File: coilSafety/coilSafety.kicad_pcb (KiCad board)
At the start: 2 copper layers, 99.1 x 99.1 mm, 22 parts, among them J1 PJ-037BH, J10 Conn_01x02_Pin, J11 Conn_01x02_Pin, J2 Screw_Terminal_01x08, J3 Screw_Terminal_01x02, J4 Screw_Terminal_01x02, J5 Screw_Terminal_01x06, J6 Screw_Terminal_01x02, J7 Conn_01x01_Pin, J8 Conn_01x08_Pin, J9 Conn_01x02_Pin, K1 AZ943-1CH-12DE

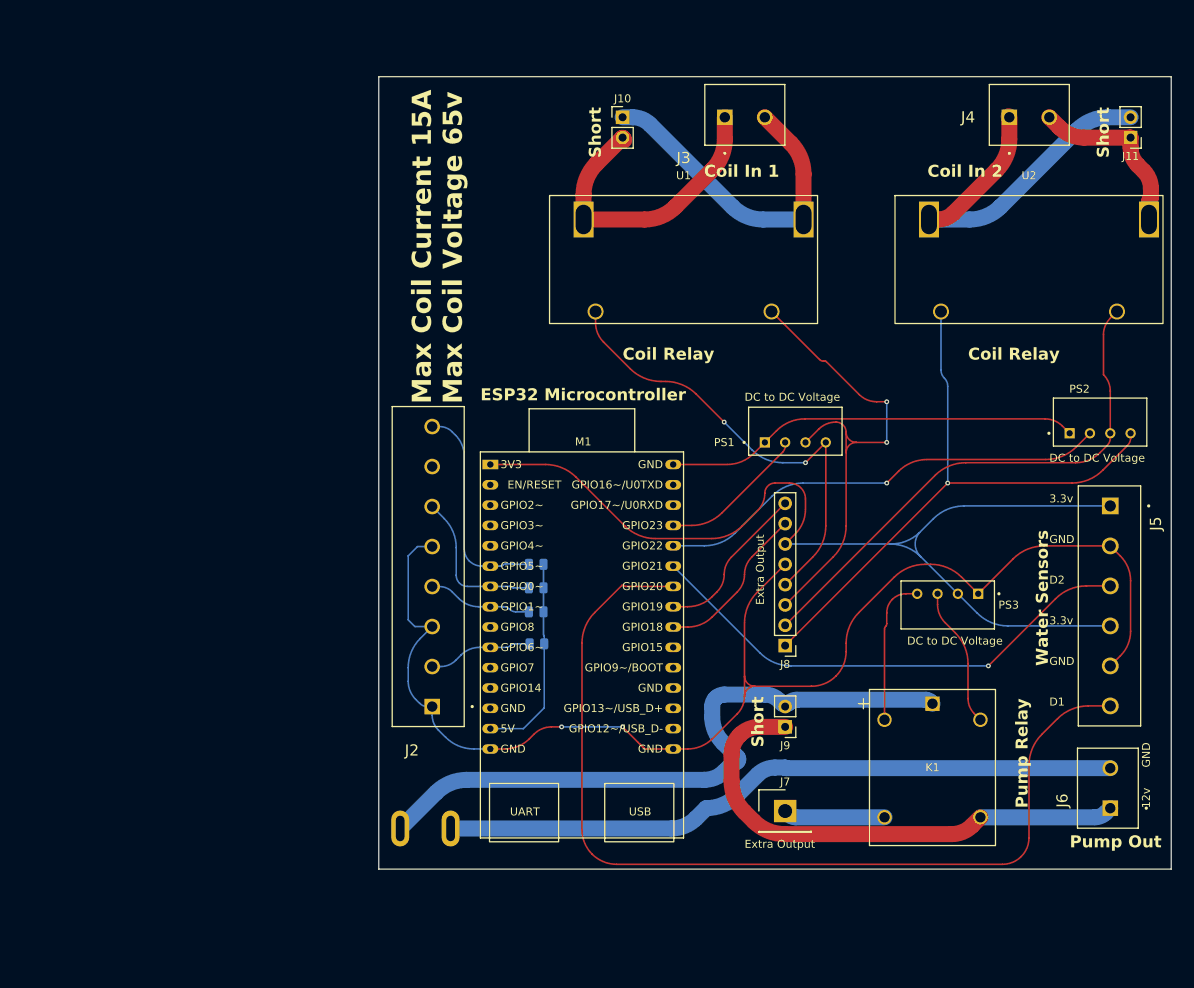
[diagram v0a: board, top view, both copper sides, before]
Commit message: Working on PCB
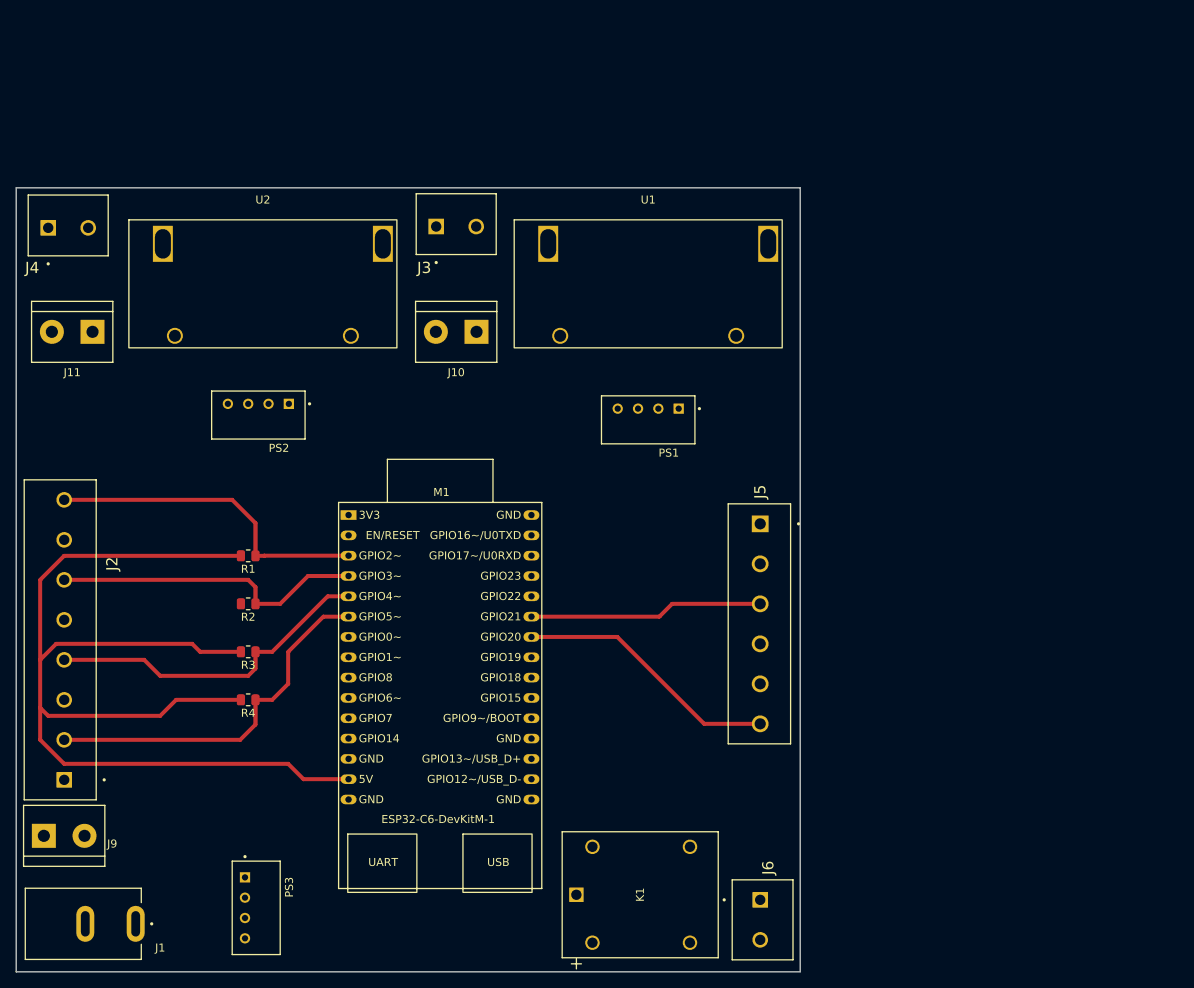
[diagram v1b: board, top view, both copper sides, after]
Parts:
- removed J7: Conn_01x01_Pin, Connector_Samtec_HPM_THT:Samtec_HPM-01-01-x-S_Straight_1x01_Pitch5.08mm
- removed J8: Conn_01x08_Pin, Connector_PinHeader_2.54mm:PinHeader_1x08_P2.54mm_Vertical
- J1, R1, R2, R3, R4: moved to F.Cu
- J10, J11, J9: footprint Connector_PinHeader_2.54mm:PinHeader_1x02_P2.54mm_Vertical -> TerminalBlock:TerminalBlock_bornier-2_P5.08mm
- M1: value ~ -> ESP32-C6-DevKitM-1
- U1, U2: value ~ -> AZDC007-1AE-12D
- moved J11 132.0 mm to (111.5, 70.0)
- moved J4 120.9 mm to (106.0, 57.0)
- moved PS2 105.2 mm to (132.3, 80.4), turned to 180 degrees
- moved U2 95.8 mm to (132.8, 64.0)
- moved PS3 94.4 mm to (132.0, 142.0), turned to -90 degrees
- moved J9 93.7 mm to (105.5, 133.0), turned to 0 degrees
- moved K1 50.5 mm to (172.0, 140.4), turned to 90 degrees
- moved J2 46.9 mm to (108.0, 126.0)
- moved J6 45.2 mm to (195.0, 141.0), turned to -90 degrees
- moved J5 43.8 mm to (195.0, 94.0)
- moved J3 38.6 mm to (154.5, 56.8)
- moved R4 36.8 mm to (131.0, 116.0), turned to 180 degrees
- moved R3 36.3 mm to (131.0, 110.0), turned to 180 degrees
- moved R2 36.1 mm to (131.0, 104.0), turned to 180 degrees
- moved R1 36.0 mm to (131.0, 98.0), turned to 180 degrees
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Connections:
- J1 pad 1: Net-(J9-Pin_2) -> Net-(J6-Pin_1)
- J1 pad 2: Net-(J6-Pin_2) -> Net-(J9-Pin_1)
- J9 pad 1: Net-(J6-Pin_1) -> Net-(J9-Pin_1)
- J9 pad 2: Net-(J9-Pin_2) -> Net-(J6-Pin_1)
- K1 pad 1: Net-(J9-Pin_2) -> Net-(J9-Pin_1)
- K1 pad 3: Net-(J7-Pin_1) -> Net-(J6-Pin_2)
- K1 pad 4: Net-(J6-Pin_1) -> Net-(J9-Pin_1)
- M1 pad 10: Net-(J2-Pin_2) -> Net-(M1-GPIO_6)
- M1 pad 22: Net-(J8-Pin_7) -> unconnected-(M1-GPIO_18-Pad22)
- M1 pad 23: Net-(J8-Pin_8) -> unconnected-(M1-GPIO_19-Pad23)
- M1 pad 3: unconnected-(M1-GPIO_2-Pad3) -> Net-(J2-Pin_8)
- M1 pad 30: Net-(PS1--VIN) -> GND
- M1 pad 4: unconnected-(M1-GPIO_3-Pad4) -> Net-(J2-Pin_6)
- M1 pad 5: unconnected-(M1-GPIO_4-Pad5) -> Net-(J2-Pin_4)
- M1 pad 6: Net-(J2-Pin_8) -> Net-(J2-Pin_2)
- M1 pad 7: Net-(J2-Pin_6) -> unconnected-(M1-GPIO_0-Pad7)
- M1 pad 8: Net-(J2-Pin_4) -> unconnected-(M1-GPIO_1-Pad8)
- PS1 pad 1: Net-(PS1--VIN) -> GND
- PS2 pad 1: Net-(PS1--VIN) -> GND
- PS3 pad 2: +3.3V -> Net-(M1-GPIO_6)
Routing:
- net GND: track 169.9 -> 0.00 mm, vias 2 -> 0
- net +3.3V: track 130.2 -> 0.00 mm
- net +5V: track 25.8 -> 139.6 mm
- net Net-(J5-Pin_6): track 122.1 -> 33.1 mm
- net Net-(J6-Pin_2): track 85.0 -> 0.00 mm
- net Net-(J9-Pin_2): track 82.2 -> 0.00 mm
- net Net-(PS2-+VOUT): track 76.2 -> 0.00 mm, vias 1 -> 0
- net Net-(PS2--VOUT): track 66.7 -> 0.00 mm
- net Net-(J6-Pin_1): track 63.9 -> 0.00 mm
- net Net-(PS1--VOUT): track 62.8 -> 0.00 mm, vias 2 -> 0
- net Net-(PS1-+VOUT): track 58.0 -> 0.00 mm, vias 2 -> 0
- net Net-(M1-GPIO_22): track 56.9 -> 0.00 mm, vias 1 -> 0
- net Net-(PS1--VIN): track 52.0 -> 0.00 mm
- net Net-(J11-Pin_2): track 48.0 -> 0.00 mm
- net Net-(J10-Pin_1): track 42.0 -> 0.00 mm
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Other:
- board size 99.1 x 99.1 mm -> 98 x 98 mm
- board text removed: "12v"
- board text removed: "3.3v"
- board text removed: "Coil In 1"
- board text removed: "Coil In 2"
- board text removed: "Coil Relay"
- board text removed: "D1"
- board text removed: "D2"
- board text removed: "DC to DC Voltage"
- board text removed: "Dr. Biedermann Electromagnet Safety Circuit"
- board text removed: "ESP32 Microcontroller"
- board text removed: "Extra Output"
- board text removed: "GND"
- board text removed: "Made By: Jackson McDowell"
- board text removed: "Max Coil Current 15A Max Coil Voltage 65v"
- board text removed: "Pump In"
- board text removed: "Pump Out"
- board text removed: "Pump Relay"
- board text removed: "Short"
- board text removed: "Water Sensors"
